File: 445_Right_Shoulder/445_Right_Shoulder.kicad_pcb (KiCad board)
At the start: 2 copper layers, 24.9 x 18 mm, 2 parts, among them J1 69167-107HLF, U1 LSM6DSMTR

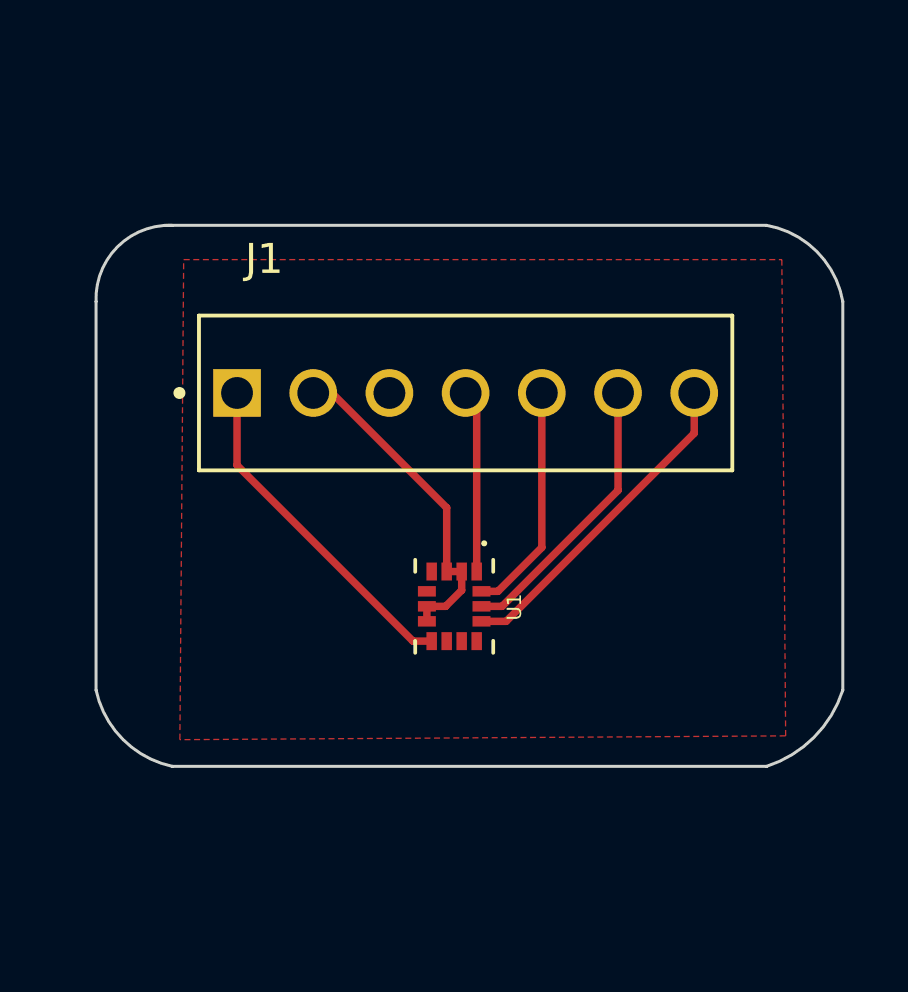
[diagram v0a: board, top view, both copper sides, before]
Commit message: Layout First Draft
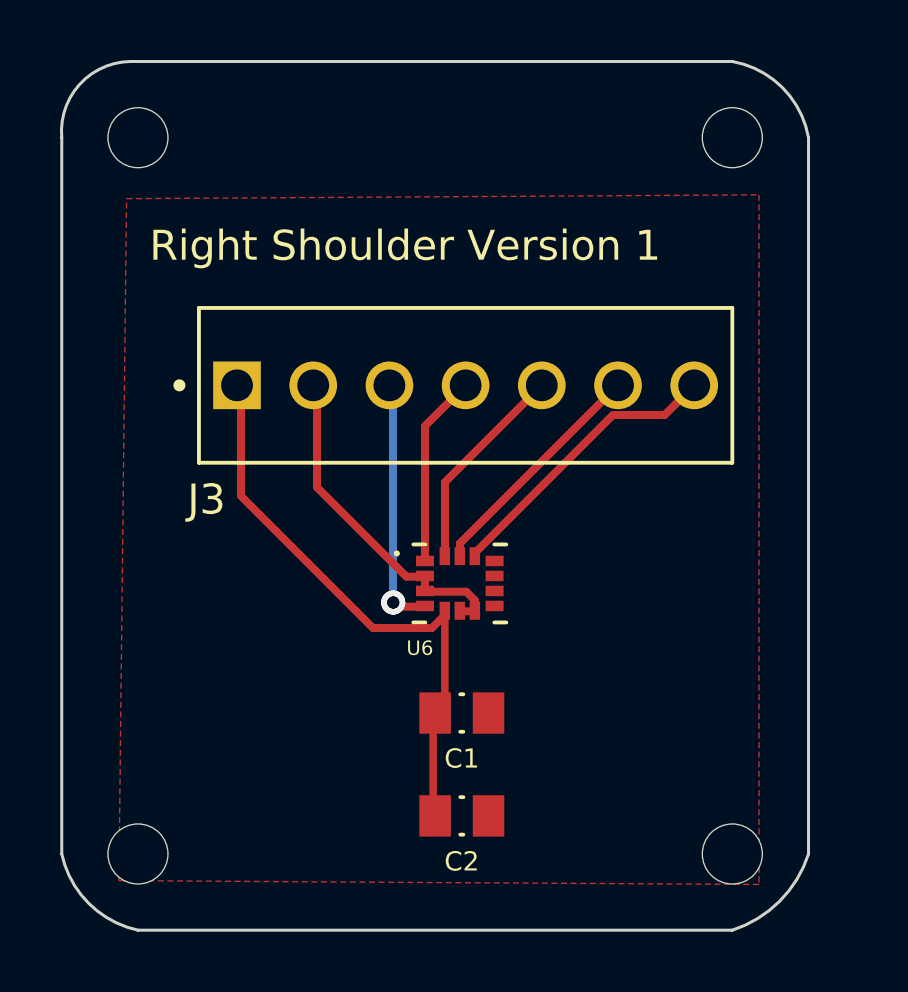
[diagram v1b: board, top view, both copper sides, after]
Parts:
- removed J1: 69167-107HLF, 69167-107HLF:AMPHENOL_69167-107HLF
- removed U1: LSM6DSMTR, LSM6DSMTR (1):PQFN50P300X250X86-14N
- added C1: 100nF, CL21F104ZAANNNC:CAPC2012X135N, F.Cu at (143.9, 94.4)
- added C2: 100nF, CL21F104ZAANNNC:CAPC2012X135N, F.Cu at (143.9, 97.8)
- added H1: MountingHole, MountingHole:MountingHole_2mm, F.Cu at (133.1, 75.2)
- added H2: MountingHole, MountingHole:MountingHole_2mm, F.Cu at (152.9, 75.2)
- added H3: MountingHole, MountingHole:MountingHole_2mm, F.Cu at (133.1, 99.1)
- added H4: MountingHole, MountingHole:MountingHole_2mm, F.Cu at (152.9, 99.1)
- added J3: 69167-107HLF, 69167-107HLF:AMPHENOL_69167-107HLF, F.Cu at (144.0, 83.4)
- added U6: LSM6DSMTR, LSM6DSMTR (1):PQFN50P300X250X86-14N, F.Cu at (143.8, 90.0)
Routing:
- net +3.3V: track 11.3 -> 32.1 mm
- net /SENSOR_1: track 0.00 -> 19.9 mm
- net /INT1_1: track 0.00 -> 17.0 mm, vias 0 -> 2
- net /CLK1: track 0.00 -> 16.2 mm
- net /MOSI_1: track 0.00 -> 14.5 mm
- net /MISO_1: track 0.00 -> 13.2 mm
- net GND: track 11.2 -> 23.0 mm
- net /CS0: track 11.0 -> 0.00 mm
- net /CLK: track 9.40 -> 0.00 mm
- net /MOSI: track 7.77 -> 0.00 mm
- net /MISO: track 6.10 -> 0.00 mm
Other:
- board size 24.9 x 18 mm -> 24.9 x 29 mm
- board text added: "Right Shoulder Version 1"
